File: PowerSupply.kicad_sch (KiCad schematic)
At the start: 84 parts, among them J14 PROG, J2 39-30-0060, J3 ENABLE, Q10 FDC5614P, Q5 BSC040N08NS5ATMA1, Q6 BSC040N08NS5ATMA1, Q7 2N7002K, Q8 NTD5867NLT4G, Q9 2N7002K, U2 ATtiny1616-S, U4 TSC2012IDT, U6 L7987, U7 AZ1117IH-3.3TRG1, U8 LM74800QDRRRQ1

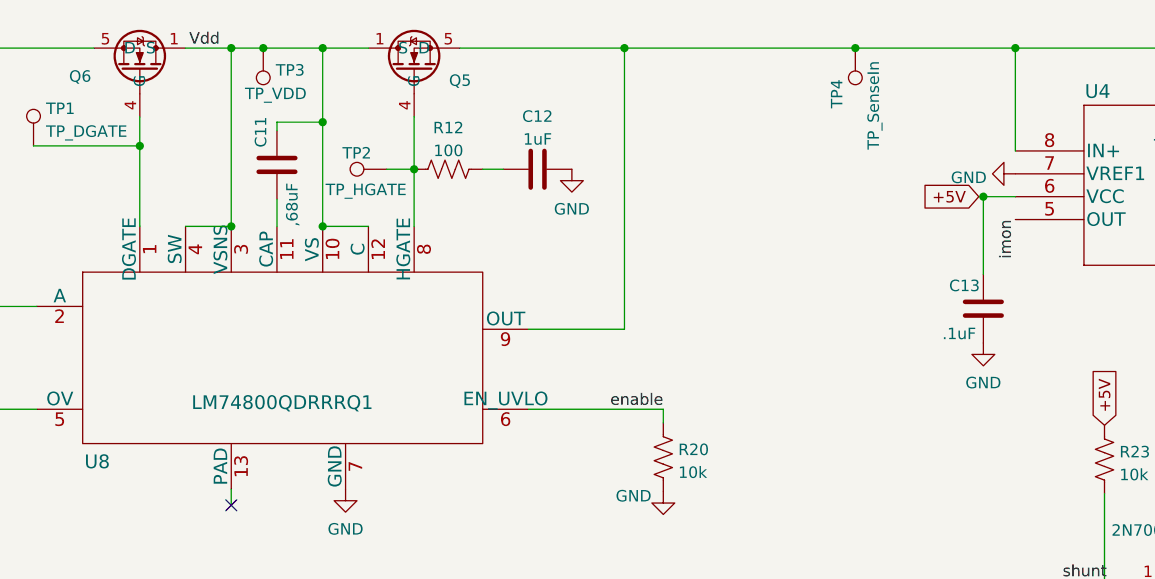
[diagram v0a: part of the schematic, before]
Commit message: removed autosave file and corrected schematic electrical rules check warnings and errors
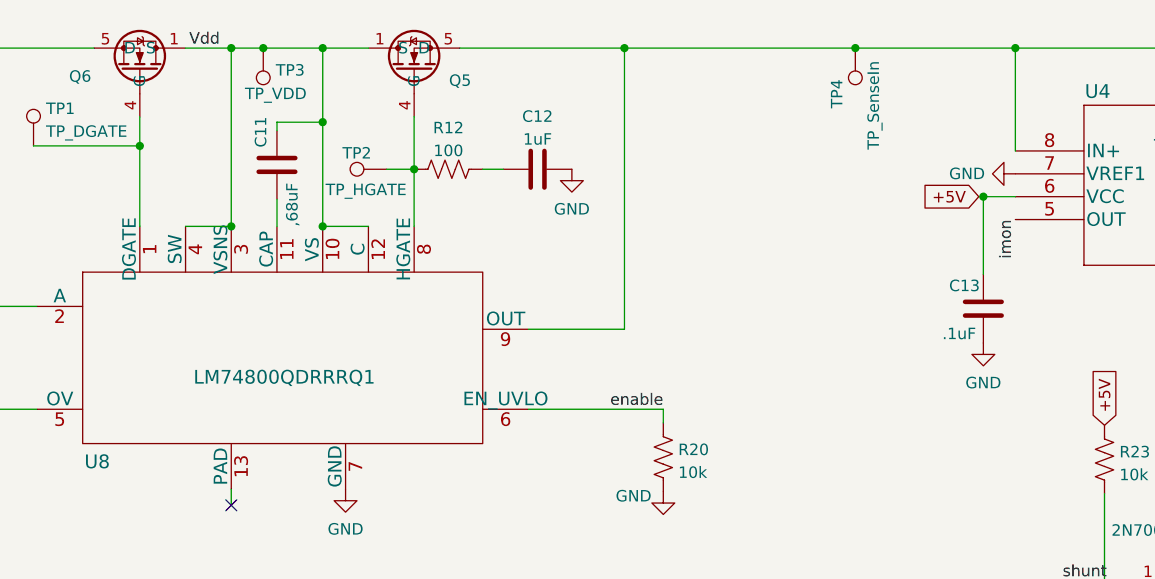
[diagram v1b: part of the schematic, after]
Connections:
- now unconnected: U8.13 (PAD)
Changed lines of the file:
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@@
     (pin "2")
+  )
+  (symbol (lib_id "power:GND") (at 187.706 30.48 270) (unit 1)
+    (in_bom yes) (on_board yes)
+    (property "Reference" "#PWR0110" (id 0) (at 181.356 30.48 0)
+      (effects (font (size 1.27 1.27)) hide)
+    )
+    (property "Value" "GND" (id 1) (at 180.34 30.48 90)
+      (effects (font (size 1.27 1.27)) (justify left))
+    )
+    (property "Footprint" "" (id 2) (at 187.706 30.48 0)
+      (effects (font (size 1.27 1.27)) hide)
+    )
+    (property "Datasheet" "" (id 3) (at 187.706 30.48 0)
+      (effects (font (size 1.27 1.27)) hide)
+    )
+    (pin "1")
   )
   (symbol (lib_id "power:GND") (at 170.688 108.712 90) (unit 1)
@@
       (effects (font (size 1.524 1.524)) (justify right))
     )
-    (property "Value" "LM74800QDRRRQ1" (id 1) (at 116.3574 55.9054 0)
+    (property "Value" "LM74800QDRRRQ1" (id 1) (at 116.586 53.086 0)
       (effects (font (size 1.524 1.524)) (justify right))
     )
@@
     (pin "12")
     (pin "13")
-    (pin "14")
-    (pin "15")
-    (pin "16")
     (pin "2")
     (pin "3")
@@
     (pin "2")
   )
-  (symbol (lib_id "power:GND") (at 187.706 30.48 270) (unit 1)
-    (in_bom yes) (on_board yes) (fields_autoplaced)
-    (property "Reference" "#PWR0110" (id 0) (at 181.356 30.48 0)
-      (effects (font (size 1.27 1.27)) hide)
-    )
-    (property "Value" "GND" (id 1) (at 184.5311 30.9138 90)
-      (effects (font (size 1.27 1.27)) (justify right))
-    )
-    (property "Footprint" "" (id 2) (at 187.706 30.48 0)
-      (effects (font (size 1.27 1.27)) hide)
-    )
-    (property "Datasheet" "" (id 3) (at 187.706 30.48 0)
-      (effects (font (size 1.27 1.27)) hide)
-    )
-    (pin "1")
-  )
   (sheet (at 183.2864 122.1232) (size 12.7 3.81) (fields_autoplaced)
